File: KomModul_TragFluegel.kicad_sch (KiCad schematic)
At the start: 36 parts, among them J1 MotorA, J2 MotorB, J5 Joystick, J6 Reserve_Klemme, SW1 Wahlschalter_Supply, SW2 Reset, U1 ATmega1284P-PU, U2 MAX485E_A, U3 MAX485E_B, Y1 16MHz

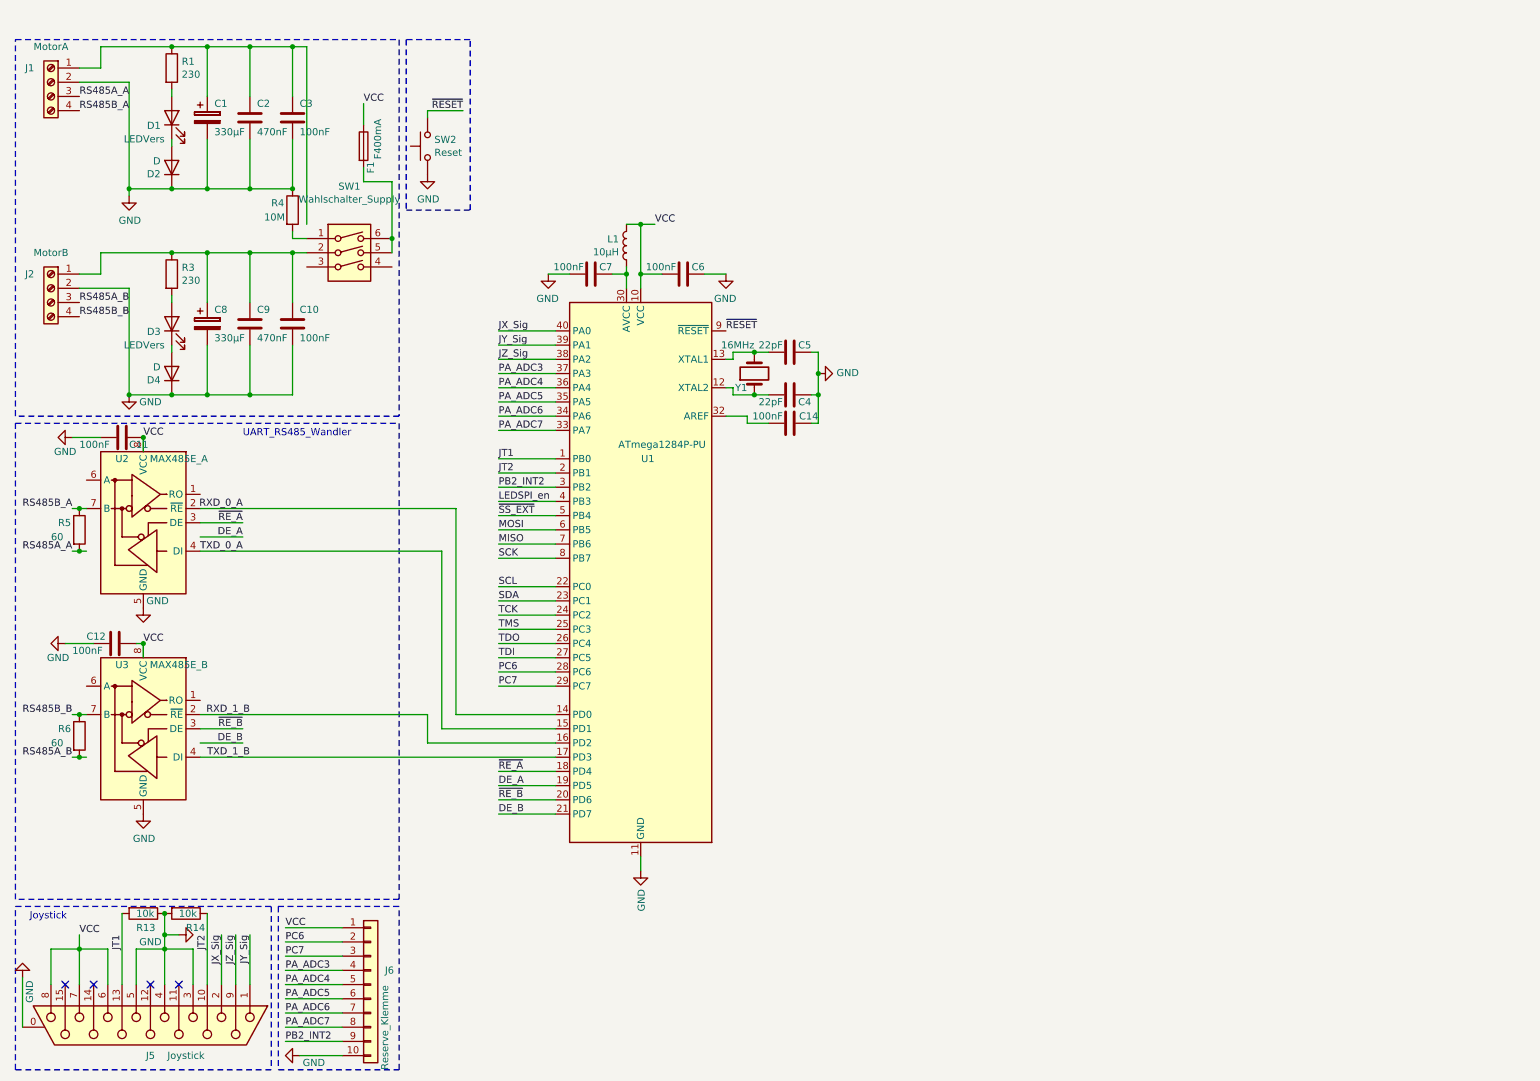
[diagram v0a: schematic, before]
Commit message: Commit vor PCB Layout
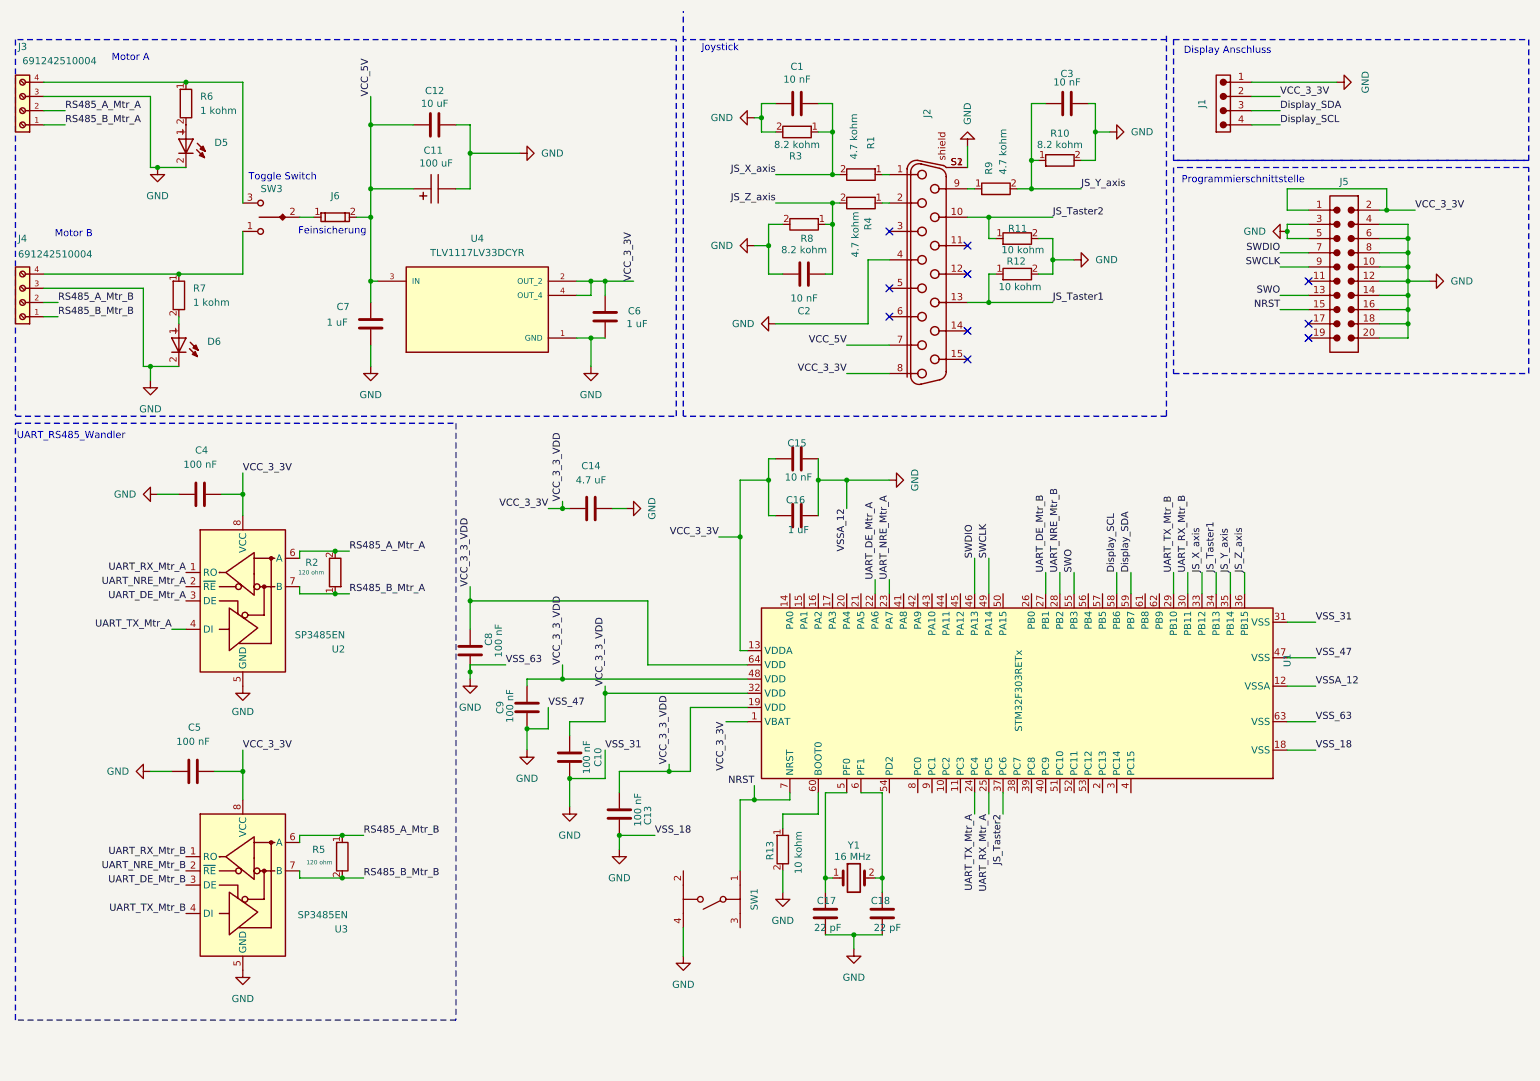
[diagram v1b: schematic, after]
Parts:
- removed C1, C8: 330µF, Capacitor_THT:CP_Radial_D12.5mm_P5.00mm, symbol Device:CP
- removed C10, C11, C12, C14, C3, C6, C7: 100nF, Capacitor_THT:C_Disc_D5.0mm_W2.5mm_P2.50mm, symbol Device:C
- removed C2, C9: 470nF, Capacitor_THT:C_Disc_D7.5mm_W5.0mm_P10.00mm, symbol Device:C
- removed C4, C5: 22pF, Capacitor_THT:C_Disc_D5.0mm_W2.5mm_P2.50mm, symbol Device:C
- removed D1, D3: LEDVers, LED_THT:LED_D5.0mm, symbol Device:LED
- removed D2, D4: D, Resistor_THT:R_Axial_DIN0207_L6.3mm_D2.5mm_P10.16mm_Horizontal, symbol Device:D
- removed F1: F400mA, MyLib:Schurter_horizontal_3101.0055, symbol Device:Fuse
- removed J1: MotorA, MyLib:TerminalBlock_RND_01.04_P_3.50mm, symbol Connector:Screw_Terminal_01x04
- removed J2: MotorB, MyLib:TerminalBlock_RND_01.04_P_3.50mm, symbol Connector:Screw_Terminal_01x04
- removed J5: Joystick, Connector_Dsub:DSUB-15_Female_Horizontal_P2.77x2.84mm_EdgePinOffset4.94mm_Housed_MountingHolesOffset7.48mm, symbol Connector:DB15_Female_MountingHoles
- removed J6: Reserve_Klemme, TerminalBlock_TE-Connectivity:TerminalBlock_TE_1-282834-0_1x10_P2.54mm_Horizontal, symbol Connector_Generic:Conn_01x10
- removed L1: 10µH, Resistor_THT:R_Axial_DIN0309_L9.0mm_D3.2mm_P12.70mm_Horizontal, symbol Device:L
- removed R1, R3: 230, Resistor_THT:R_Axial_DIN0207_L6.3mm_D2.5mm_P10.16mm_Horizontal, symbol Device:R
- removed R13, R14: 10k, Resistor_THT:R_Axial_DIN0207_L6.3mm_D2.5mm_P10.16mm_Horizontal, symbol Device:R
- removed R4: 10M, Resistor_THT:R_Axial_DIN0207_L6.3mm_D2.5mm_P10.16mm_Horizontal, symbol Device:R
- removed R5, R6: 60, Resistor_THT:R_Axial_DIN0207_L6.3mm_D2.5mm_P10.16mm_Horizontal, symbol Device:R
- removed SW1: Wahlschalter_Supply, Button_Switch_THT:SW_DIP_SPSTx03_Slide_6.7x9.18mm_W7.62mm_P2.54mm_LowProfile, symbol Switch:SW_DIP_x03
- removed SW2: Reset, Button_Switch_THT:SW_PUSH_6mm_H4.3mm, symbol Switch:SW_Push
- removed U1: ATmega1284P-PU, Package_DIP:DIP-40_W15.24mm, symbol MCU_Microchip_ATmega:ATmega1284P-PU
- removed U2: MAX485E_A, Package_DIP:DIP-8_W7.62mm_Socket, symbol Interface_UART:MAX485E
- removed U3: MAX485E_B, Package_DIP:DIP-8_W7.62mm_Socket, symbol Interface_UART:MAX485E
- removed Y1: 16MHz, Crystal:Crystal_HC49-4H_Vertical, symbol Device:Crystal
- added C1, C15, C2, C3: 10 nF, Capacitor_SMD_Wurth:C_Wurth_WCAP-CSGP-1206_H0.8, symbol symbols:1206_H0.8_885012208026
- added C10, C13, C8, C9: 100 nF, Capacitor_SMD_Wurth:C_Wurth_WCAP-CSGP-1206_H0.8, symbol symbols:1206_H0.8_885012208030
- added C11: 100 uF, Capacitor_THT_Wurth:CP_Wurth_WCAP-PT5H-P2.5D6.3L11, symbol symbols:P2.5D6.3L11_870235373001
- added C12: 10 uF, Capacitor_SMD_Wurth:C_Wurth_WCAP-CSGP-1206_H1.6, symbol symbols:1206_H1.6_885012208041
- added C14: 4.7 uF, Capacitor_SMD_Wurth:C_Wurth_WCAP-CSGP-1206_H1.6, symbol symbols:1206_H1.6_885012208040
- added C16, C6, C7: 1 uF, Capacitor_SMD_Wurth:C_Wurth_WCAP-CSGP-1206_H1.15, symbol symbols:1206_H1.15_885012208036
- added C17, C18: 22 pF, Capacitor_SMD_Wurth:C_Wurth_WCAP-CSGP-1206_H0.8, symbol symbols:1206_H0.8_885012008011
- added C4, C5: 100 nF, Capacitor_SMD_Wurth:C_Wurth_WCAP-CSGP-0805_H0.8_R, symbol Capacitor_Wurth_WCAP-CSGP:0805_H0.8_R_885012207072
- added D5, D6: 5mmWOS_151051RS11000, LED_THT_Wurth:D_Wurth_WL-TMRC-5mmWOS, symbol LED_Wurth_WL-TMRC:5mmWOS_151051RS11000
- added J1: 66100411622, Connector_THT_Wurth:J_Wurth_WR-WTB_66100411622, symbol symbols:66100411622
- added J2: 618015231121, Connector_THT_Wurth:J_Wurth_WR-DSUB_618015231121, symbol symbols:618015231121
- added J3, J4: 691242510004, Terminal_Wuerth_Block:691242510004, symbol 691242510004:691242510004
- added J5: 612020235121, Connector_THT_Wurth:J_Wurth_WR-BHD_612020235121, symbol symbols:612020235121
- added J6: 696106003002, Connector_THT_Wurth:J_Wurth_WR-FSH_696106003002, symbol symbols:696106003002
- added R1, R4, R9: 4.7 kohm, Resistor_SMD_Wurth:R_Wurth_WRIS-RSKS-1206_R, symbol symbols:1206_R_560112132020
- added R10, R3, R8: 8.2 kohm, Resistor_SMD_Wurth:R_Wurth_WRIS-RSKS-1206_R, symbol symbols:1206_R_560112132051
- added R11, R12, R13: 10 kohm, Resistor_SMD_Wurth:R_Wurth_WRIS-RSKS-1206_R, symbol symbols:1206_R_560112132018
- added R2, R5: 120 ohm, Resistor_SMD_Wurth:R_Wurth_WRIS-RSKS-1210_R, symbol Resistor_Wurth_WRIS-RSKS:1210_R_560112140009
- added R6, R7: 1 kohm, Resistor_SMD_Wurth:R_Wurth_WRIS-RSKS-1206_R, symbol symbols:1206_R_560112132038
- added SW1: 430182080816, Switch_SMD_Wurth:SW_Wurth_WS-TASV_430182080816, symbol symbols:430182080816
- added SW3: 472123010111, Switch_THT_Wurth:SW_Wurth_WS-TOTV_472123010111, symbol symbols:472123010111
- added U1: STM32F303RETx, Package_QFP:LQFP-64_10x10mm_P0.5mm, symbol MCU_ST_STM32F3:STM32F303RETx
- added U2, U3: SP3485EN, Package_SO:SOIC-8_3.9x4.9mm_P1.27mm, symbol Interface_UART:SP3485EN
- added U4: TLV1117LV33DCYR, MyLib:VREG_TLV1117LV33DCYR, symbol TLV1117LV33DCYR:TLV1117LV33DCYR
- added Y1: 16 MHz, Crystal_THT_Wurth:Y_Wurth_WE-XTAL_Quartz-HC49-4H, symbol symbols:HC49-4H_830058383B
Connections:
- net GND: now also C1.2, C10.1, C11.2, C12.1, C13.1, C14.2, C15.2, C16.1, C17.2, C18.2, C2.1, C3.2, C4.1, C5.1, C6.2, C7.2, C8.1, C9.2, D5.2 (-), D6.2 (-), J1.1, J2.4, J2.S1 (SHIELD), J2.S2 (SHIELD), J3.3, J4.3, J5.10, J5.12, J5.14, J5.16, J5.18, J5.20, J5.3, J5.4, J5.5, J5.6, J5.8, R10.2, R11.2, R12.2, R13.2, R3.2, R8.2, SW1.4, U1.12 (VSSA), U1.18 (VSS), U1.31 (VSS), U1.47 (VSS), U1.63 (VSS), U2.5 (GND), U3.5 (GND), U4.1 (GND)
- new net: J3.4, R6.1, SW3.3
- new net: C17.1, U1.5 (PF0), Y1.1
- new net: C18.1, U1.6 (PF1), Y1.2
- new net: R13.1, U1.60 (BOOT0)
- new net: D5.1 (+), R6.2
- new net: J4.4, R7.1, SW3.1
- new net: J6.1, SW3.2
- new net: J2.2, R4.1
- new net: J2.9, R9.1
- new net: J2.1, R1.1
- new net: D6.1 (+), R7.2
- new net Display_SCL: J1.4, U1.58 (PB6)
- new net Display_SDA: J1.3, U1.59 (PB7)
- new net JS_Taster1: J2.13, R12.1, U1.34 (PB13)
- new net JS_Taster2: J2.10, R11.1, U1.37 (PC6)
- new net JS_X_axis: C1.1, R1.2, R3.1, U1.33 (PB12)
- new net JS_Y_axis: C3.1, R10.1, R9.2, U1.35 (PB14)
- new net JS_Z_axis: C2.2, R4.2, R8.1, U1.36 (PB15)
- new net NRST: J5.15, SW1.1, U1.7 (NRST)
- new net RS485_A_Mtr_A: J3.2, R2.2, U2.6 (A)
- new net RS485_A_Mtr_B: J4.2, R5.1, U3.6 (A)
- new net RS485_B_Mtr_A: J3.1, R2.1, U2.7 (B)
- new net RS485_B_Mtr_B: J4.1, R5.2, U3.7 (B)
- new net SWCLK: J5.9, U1.49 (PA14)
- new net SWDIO: J5.7, U1.46 (PA13)
- new net SWO: J5.13, U1.55 (PB3)
- new net UART_DE_Mtr_A: U1.22 (PA6), U2.3 (DE)
- new net UART_DE_Mtr_B: U1.27 (PB1), U3.3 (DE)
- new net UART_NRE_Mtr_A: U1.23 (PA7), U2.2 (~{RE})
- new net UART_NRE_Mtr_B: U1.28 (PB2), U3.2 (~{RE})
- new net UART_RX_Mtr_A: U1.25 (PC5), U2.1 (RO)
- new net UART_RX_Mtr_B: U1.30 (PB11), U3.1 (RO)
- new net UART_TX_Mtr_A: U1.24 (PC4), U2.4 (DI)
- new net UART_TX_Mtr_B: U1.29 (PB10), U3.4 (DI)
- new net VCC_3_3V: C10.2, C13.2, C14.1, C15.1, C16.2, C4.2, C5.2, C6.1, C8.2, C9.1, J1.2, J2.8, J5.1, J5.2, U1.1 (VBAT), U1.13 (VDDA), U1.19 (VDD), U1.32 (VDD), U1.48 (VDD), U1.64 (VDD), U2.8 (VCC), U3.8 (VCC), U4.2 (OUT_2), U4.4 (OUT_4)
- new net VCC_5V: C11.1, C12.2, C7.1, J2.7, J6.2, U4.3 (IN)
- no-connect marks 4 -> 10
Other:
- note added: "Display Anschluss"
- note added: "Feinsicherung"
- note added: "Motor A"
- note added: "Motor B"
- note added: "Programmierschnittstelle"
- note added: "Toggle Switch"
- title: Kommunikationsmodul Tragflügelboot -> Kommunikationsmodul Tragflügelboot Joystick
